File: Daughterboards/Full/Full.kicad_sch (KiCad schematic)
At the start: 19 parts

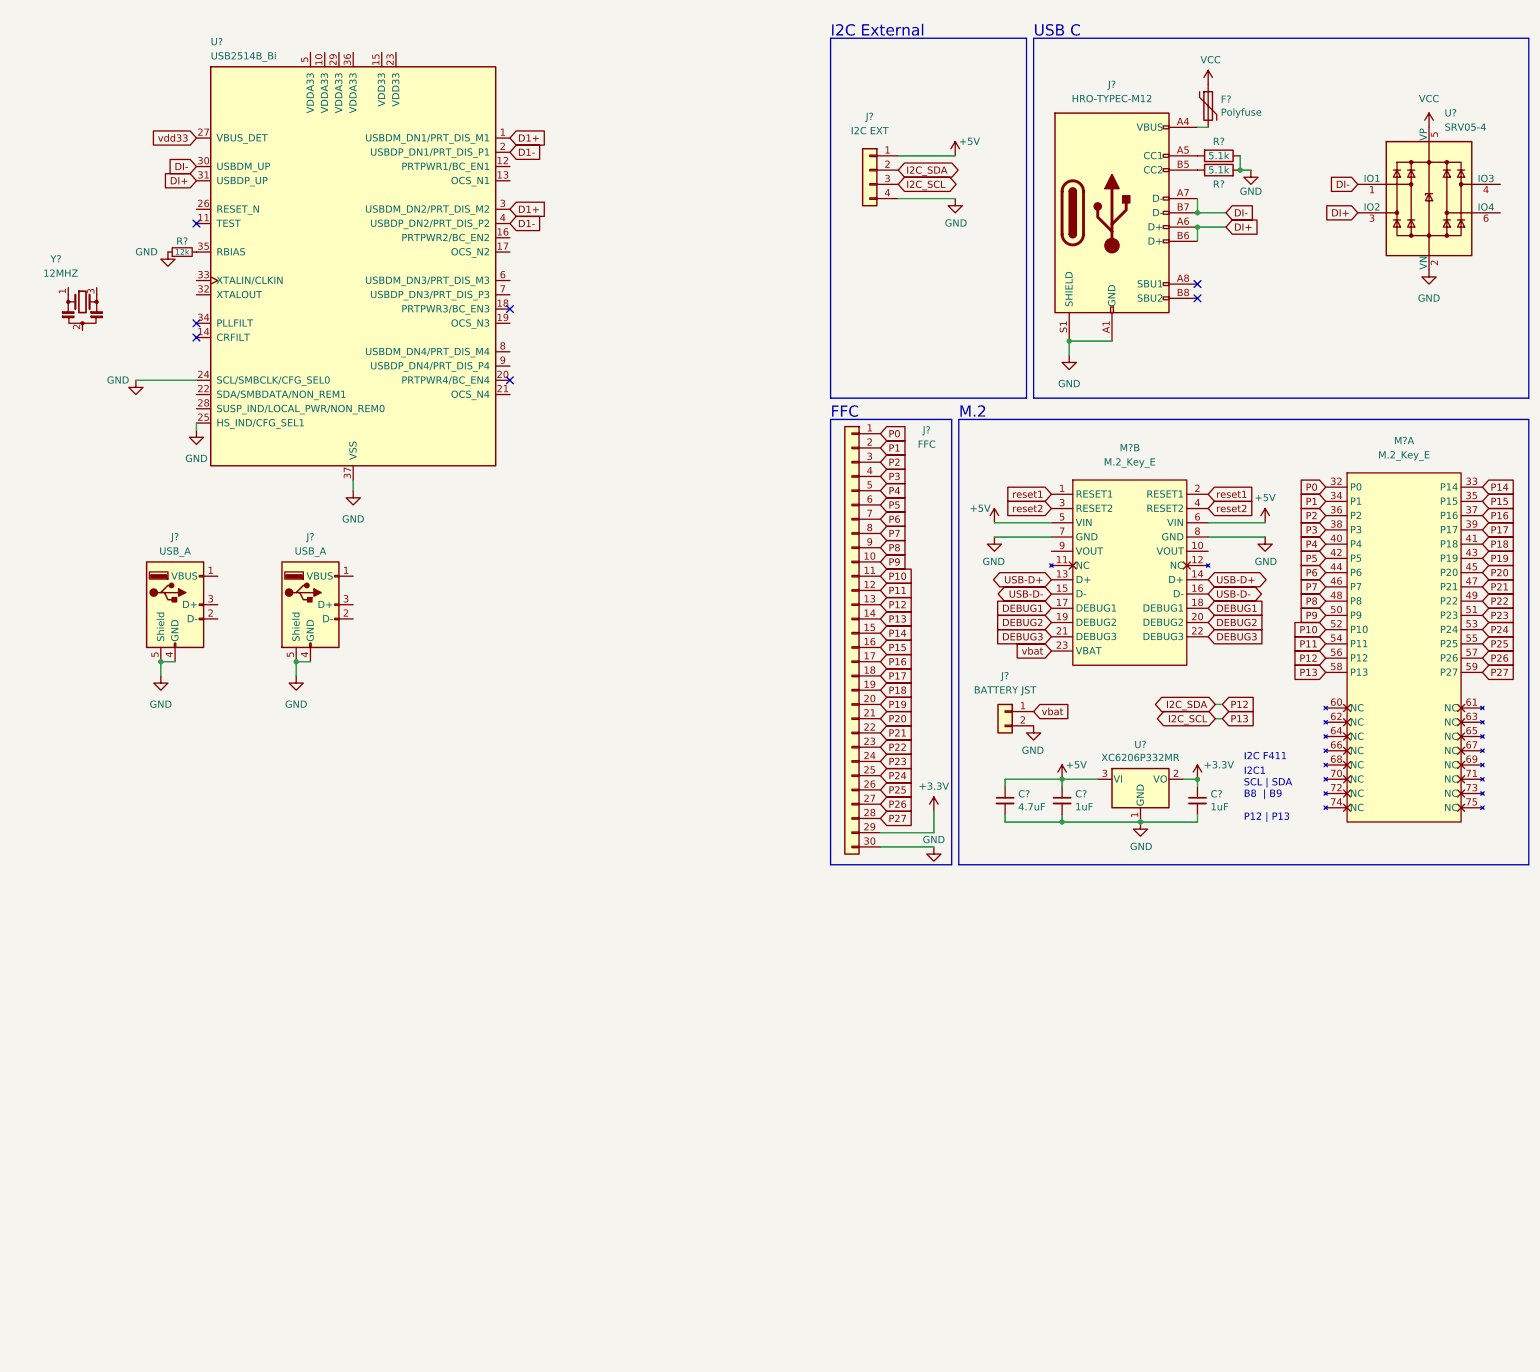
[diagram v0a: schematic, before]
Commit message: major progress on the full db
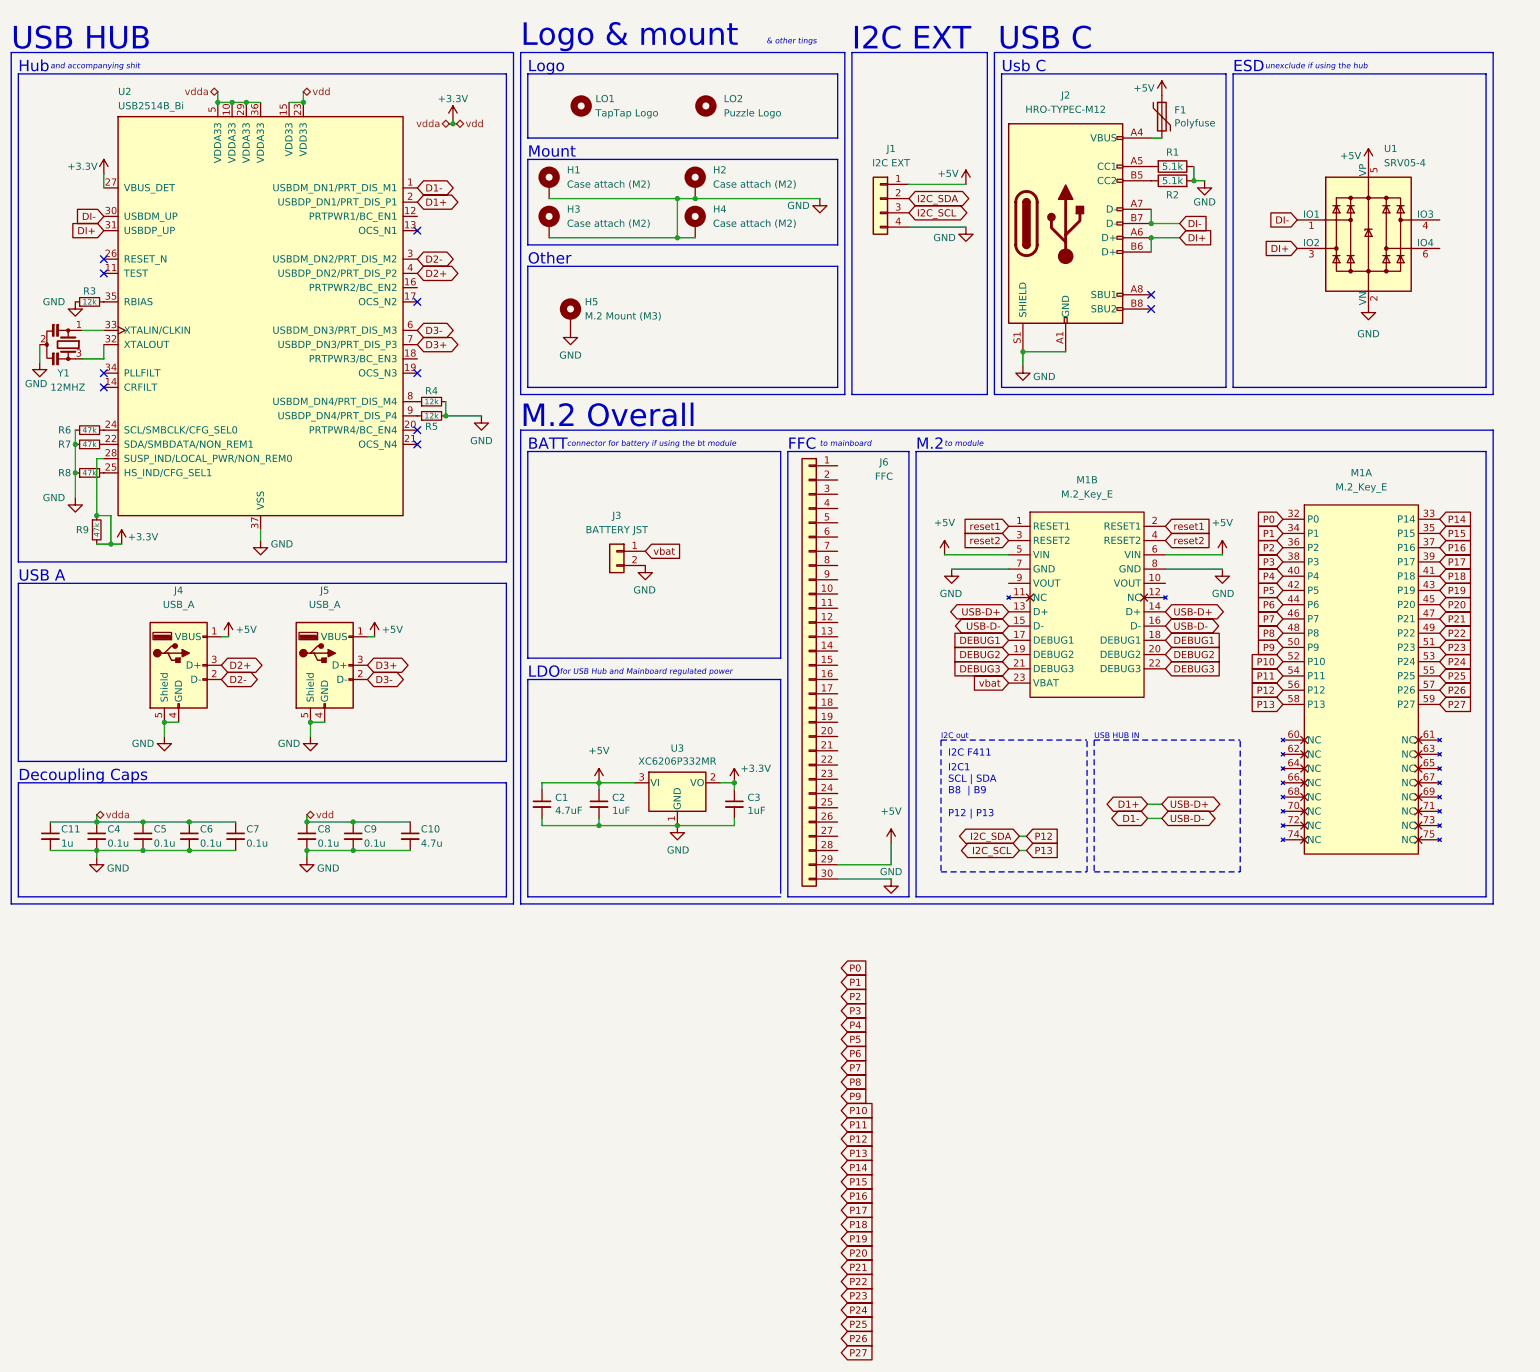
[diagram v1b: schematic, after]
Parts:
- removed J? (x2): USB_A, Connector_USB:USB_A_Stewart_SS-52100-001_Horizontal, symbol Connector:USB_A
- added C10: 4.7u, Capacitor_SMD:C_0402_1005Metric, symbol Device:C_Small
- added C11: 1u, Capacitor_SMD:C_0402_1005Metric, symbol Device:C_Small
- added C4, C5, C6, C7, C8, C9: 0.1u, Capacitor_SMD:C_0402_1005Metric, symbol Device:C_Small
- added H1, H2, H3, H4: Case attach (M2), MountingHole:MountingHole_2.2mm_M2_Pad, symbol Mechanical:MountingHole_Pad
- added H5: M.2 Mount (M3), MountingHole:MountingHole_3.2mm_M3_DIN965_Pad, symbol Mechanical:MountingHole_Pad
- added J4, J5: USB_A, Connector_USB:USB_A_Stewart_SS-52100-001_Horizontal, symbol Connector:USB_A
- added LO1: TapTap Logo, LogoSmall:tt_4mm, symbol Mechanical:MountingHole
- added LO2: Puzzle Logo, LogoSmall:LogoSmall, symbol Mechanical:MountingHole
- added R4, R5: 12k, Resistor_SMD:R_0402_1005Metric, symbol Device:R_Small
- added R6, R7, R8, R9: 47k, Resistor_SMD:R_0402_1005Metric, symbol Device:R_Small
- J1: renamed from J?; footprint Connector:Banana_Jack_1Pin -> Connector-pat-various:Magnetic Pogo 4 pin
- J2: renamed from J?; footprint (none) -> Connector_USB:USB_C_Receptacle_HRO_TYPE-C-31-M-12
- J3: renamed from J?; footprint (none) -> Connector_JST:JST_PH_S2B-PH-SM4-TB_1x02-1MP_P2.00mm_Horizontal
- J6: renamed from J?; footprint (none) -> Connector-pat-various:100519223010ELF
- M1: renamed from M?; footprint (none) -> m2ngff:m2-bracket-key-e
- R1, R2: renamed from R?; footprint Resistor_SMD:R_0805_2012Metric -> Resistor_SMD:R_0402_1005Metric
- R3: renamed from R?; footprint (none) -> Resistor_SMD:R_0402_1005Metric
- U2: renamed from U?; footprint Package_DFN_QFN:QFN-36-1EP_6x6mm_P0.5mm_EP3.7x3.7mm -> Package_DFN_QFN:QFN-36-1EP_6x6mm_P0.5mm_EP3.7x3.7mm_ThermalVias
- Y1: renamed from Y?; footprint (none) -> Crystal:Resonator_SMD_Murata_CSTxExxV-3Pin_3.0x1.1mm
- gave numbers to parts that had none: 6
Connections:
- net USB-D+ is gone; now on net D1+: M1.13 (D+), M1.14 (D+)
- net USB-D- is gone; now on net D1-: M1.15 (D-), M1.16 (D-)
- net VCC is gone; now on net +5V: F1.1, U1.5 (VP)
- net vdd33 is gone; now on net +3V3: U2.27 (VBUS_DET)
- net +3V3: now also U2.10 (VDDA33), U2.15 (VDD33), U2.23 (VDD33), U2.28 (SUSP_IND/LOCAL_PWR/NON_REM0), U2.29 (VDDA33), U2.36 (VDDA33), U2.5 (VDDA33), C10.1, C11.1, C4.1, C5.1, C6.1, C7.1, C8.1, C9.1, R9.1, R9.2; no longer J6.29 (Pin_29)
- net +5V: now also J6.29 (Pin_29), J4.1 (VBUS), J5.1 (VBUS)
- net D1+: now also U2.2 (USBDP_DN1/PRT_DIS_P1); no longer U2.1 (USBDM_DN1/PRT_DIS_M1), U2.3 (USBDM_DN2/PRT_DIS_M2)
- net D1-: now also U2.1 (USBDM_DN1/PRT_DIS_M1); no longer U2.2 (USBDP_DN1/PRT_DIS_P1), U2.4 (USBDP_DN2/PRT_DIS_P2)
- net GND: now also Y1.2, C10.2, C11.2, C4.2, C5.2, C6.2, C7.2, C8.2, C9.2, H1.1, H2.1, H3.1, H4.1, H5.1, J4.4 (GND), J4.5 (Shield), J5.4 (GND), J5.5 (Shield), R4.2, R5.2, R6.1, R7.1, R8.1; no longer U2.24 (SCL/SMBCLK/CFG_SEL0), U2.25 (HS_IND/CFG_SEL1)
- net I2C_SCL: no longer J6.14 (Pin_14)
- net I2C_SDA: no longer J6.13 (Pin_13)
- net P0: no longer J6.1 (Pin_1)
- net P1: no longer J6.2 (Pin_2)
- net P10: no longer J6.11 (Pin_11)
- net P11: no longer J6.12 (Pin_12)
- net P14: no longer J6.15 (Pin_15)
- net P15: no longer J6.16 (Pin_16)
- net P16: no longer J6.17 (Pin_17)
- net P17: no longer J6.18 (Pin_18)
- net P18: no longer J6.19 (Pin_19)
- net P19: no longer J6.20 (Pin_20)
- net P2: no longer J6.3 (Pin_3)
- net P20: no longer J6.21 (Pin_21)
- net P21: no longer J6.22 (Pin_22)
- net P22: no longer J6.23 (Pin_23)
- net P23: no longer J6.24 (Pin_24)
- net P24: no longer J6.25 (Pin_25)
- net P25: no longer J6.26 (Pin_26)
- net P26: no longer J6.27 (Pin_27)
- net P27: no longer J6.28 (Pin_28)
- net P3: no longer J6.4 (Pin_4)
- net P4: no longer J6.5 (Pin_5)
- net P5: no longer J6.6 (Pin_6)
- net P6: no longer J6.7 (Pin_7)
- net P7: no longer J6.8 (Pin_8)
- net P8: no longer J6.9 (Pin_9)
- net P9: no longer J6.10 (Pin_10)
- net at U2.22 (SDA/SMBDATA/NON_REM1): now also R7.2
- net at U2.32 (XTALOUT): now also Y1.3
- net at U2.33 (XTALIN/CLKIN): now also Y1.1
- net D3-: now reaches U2.6 (USBDM_DN3/PRT_DIS_M3)
- net D3-: now also J5.2 (D-)
- net D3+: now reaches U2.7 (USBDP_DN3/PRT_DIS_P3)
- net D3+: now also J5.3 (D+)
- net at U2.8 (USBDM_DN4/PRT_DIS_M4): now also R4.1
- net at U2.9 (USBDP_DN4/PRT_DIS_P4): now also R5.1
- new net: R6.2, U2.24 (SCL/SMBCLK/CFG_SEL0)
- new net: R8.2, U2.25 (HS_IND/CFG_SEL1)
- new net D2+: J4.3 (D+), U2.4 (USBDP_DN2/PRT_DIS_P2)
- new net D2-: J4.2 (D-), U2.3 (USBDM_DN2/PRT_DIS_M2)
- no-connect marks 7 -> 11
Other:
- note added: "& other tings"
- note added: "BATT"
- note added: "Decoupling Caps"
- note added: "ESD"
- note added: "Hub"
- note added: "I2C EXT"
- note added: "I2C out"
- note added: "LDO"
- note added: "Logo"
- note added: "Logo & mount"
- note added: "M.2 Overall"
- note added: "Mount"
- note added: "Other"
- note added: "USB A"
- note added: "USB HUB"
- note added: "USB HUB IN"
- note added: "Usb C"
- note added: "and accompanying shit"
- note added: "connector for battery if using the bt module"
- note added: "for USB Hub and Mainboard regulated power"
- note added: "to mainboard"
- note added: "to module"
- note added: "unexclude if using the hub"
- note removed: "I2C External"
- company: (none) -> TapTap
- title: (none) -> Full
- moved on the sheet: C1, C2, C3, F1, J1, J2, J3, J6, M1A, M1B, R1, R2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
